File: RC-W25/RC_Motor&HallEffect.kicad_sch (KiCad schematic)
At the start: 10 parts, among them P1 CONN HEADER SMD R/A 2POS 2MM, Q1 NMOS, U3 TMAG5253, U4 TMAG5253, U6 PTS645SM43SMTR92LFS

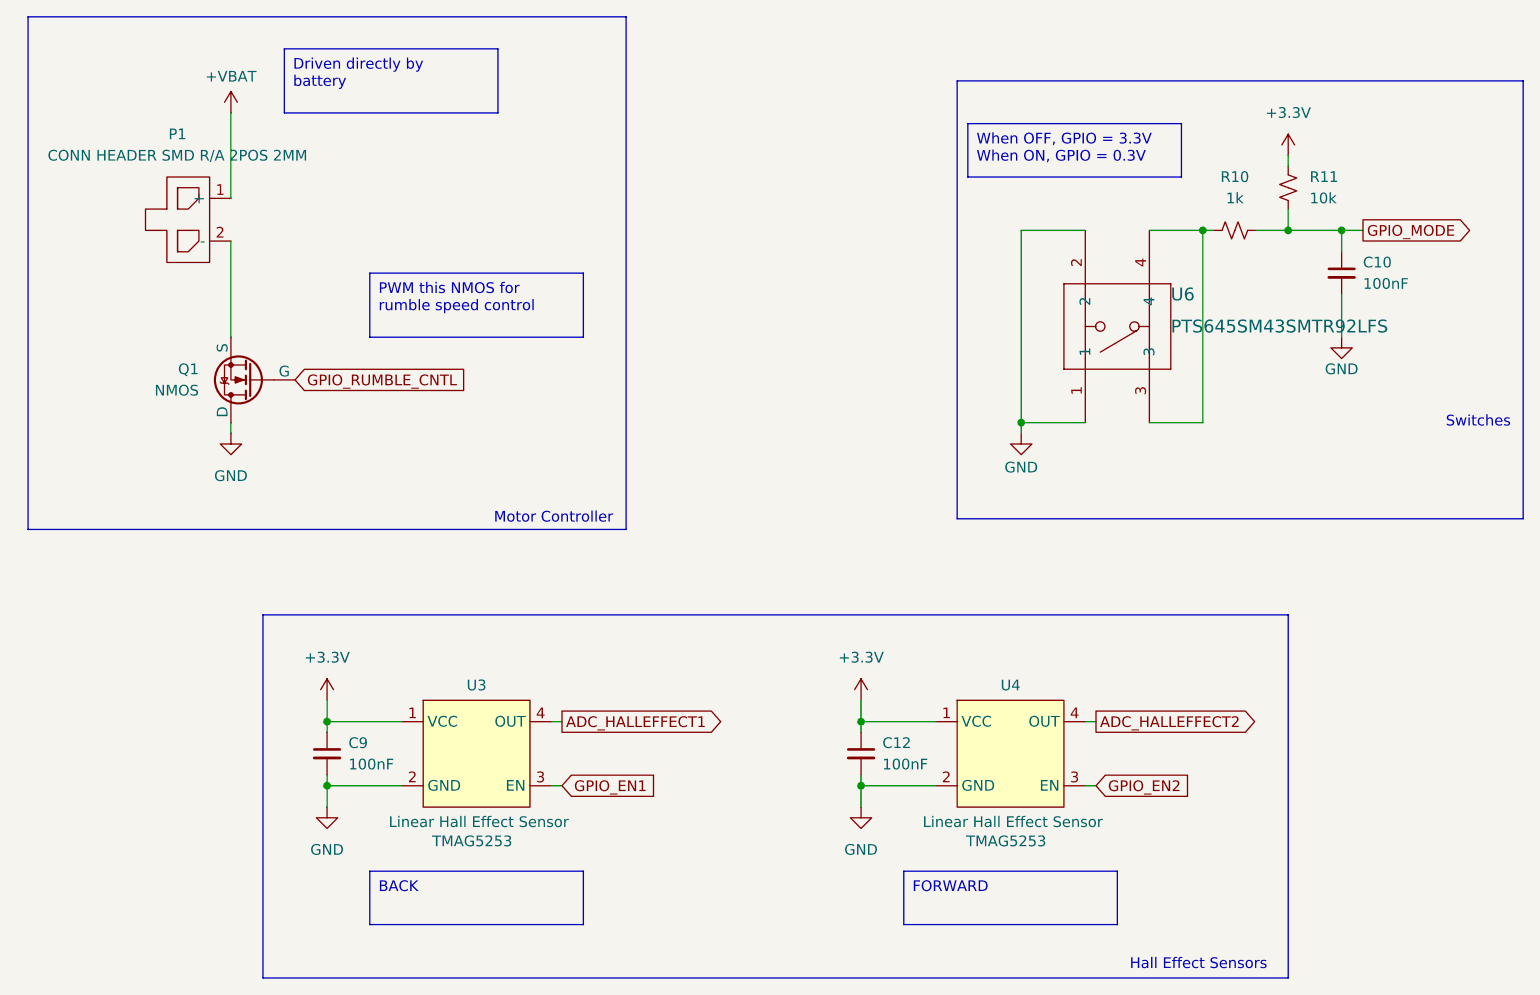
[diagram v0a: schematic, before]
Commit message: Almost Finalized Schematic
Still need to spec out buttons and jst conn
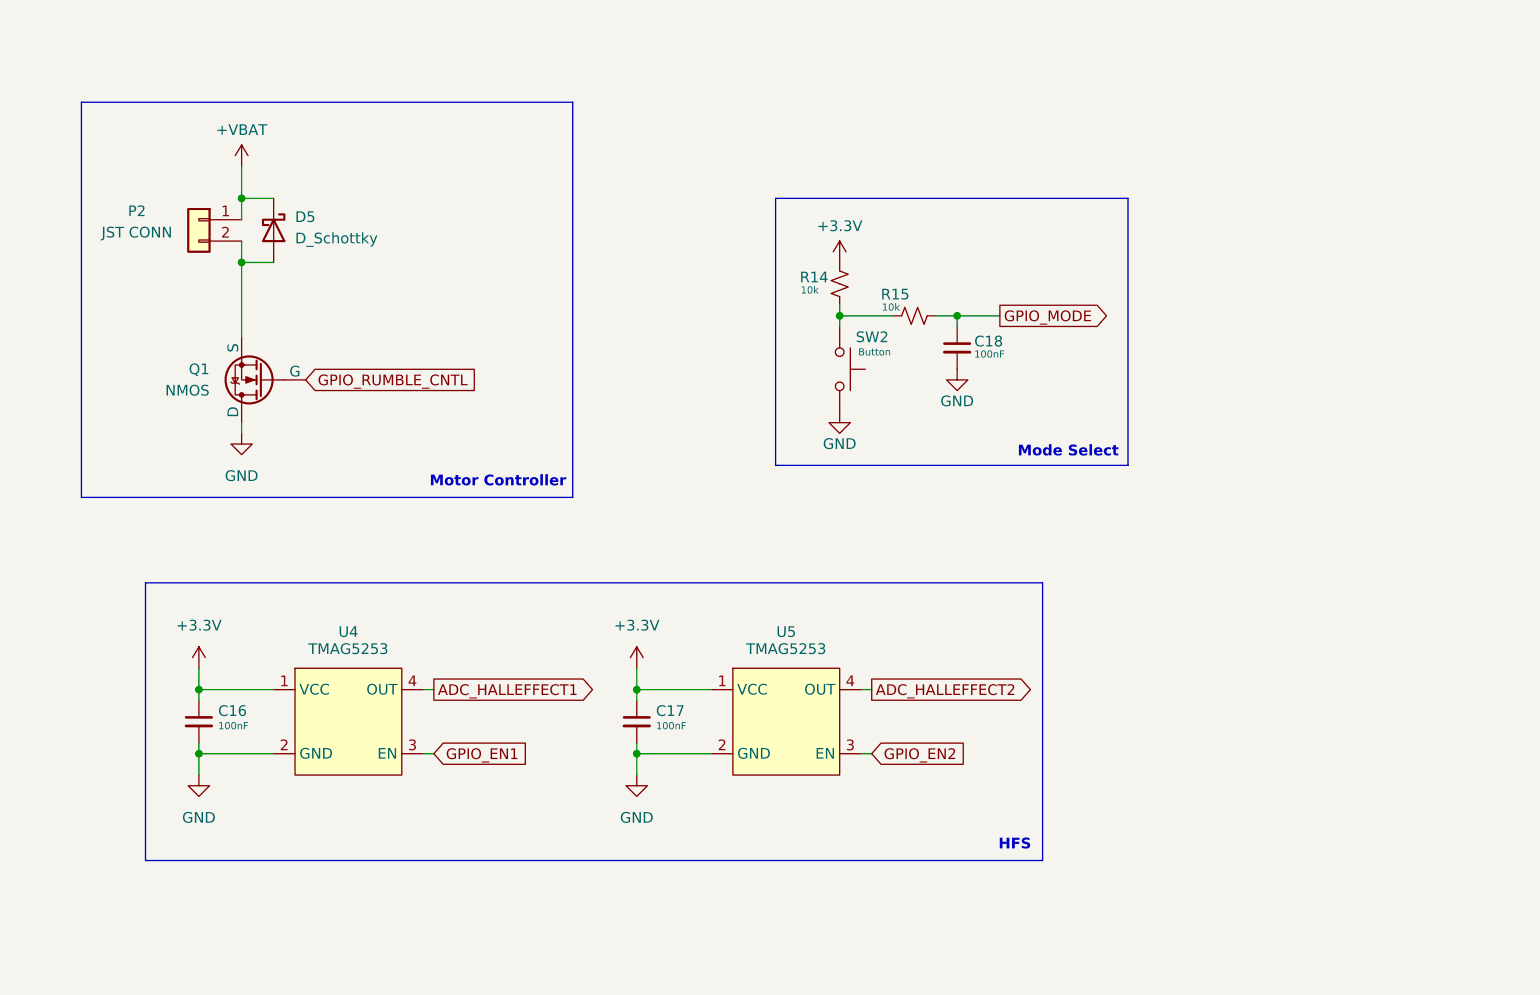
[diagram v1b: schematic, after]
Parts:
- removed C10, C12: 100nF, Capacitor_SMD:C_0603_1608Metric, symbol Device:C_Small
- removed P1: CONN HEADER SMD R/A 2POS 2MM, Library:CONN02_502352_MOL, symbol New_Library:DuraClik_CONN_HEADER_SMD_R/A_2POS_2MM
- removed R10: 1k, Resistor_SMD:R_0603_1608Metric, symbol Device:R_Small_US
- removed R11: 10k, Resistor_SMD:R_0603_1608Metric, symbol Device:R_Small_US
- removed U4: TMAG5253, Library:X2SON4_DMR_TEX-M, symbol New_Library_0:TMAG5253_Linear_Hall_Effect_Sensor
- removed U6: PTS645SM43SMTR92LFS, Library:SWITCH_43SMTR92LFS, symbol New_Library_5:PTS645SM43SMTR92LFS
- added C17, C18: 100nF, Capacitor_SMD:C_0402_1005Metric, symbol Device:C_Small
- added D5: D_Schottky, Diode_SMD:D_SOD-123, symbol Device:D_Schottky
- added P2: JST CONN, Library:CONN02_502352_MOL, symbol Connector_Generic:Conn_01x02
- added R14, R15: 10k, Resistor_SMD:R_0402_1005Metric, symbol Device:R_Small_US
- added SW2: Button, symbol Switch:SW_Push
- added U5: TMAG5253, Library:X2SON4_DMR_TEX-M, symbol New_Library_0:TMAG5253_Linear_Hall_Effect_Sensor
- C16: renamed from C9; footprint Capacitor_SMD:C_0603_1608Metric -> Capacitor_SMD:C_0402_1005Metric; LCSC# (none) -> C22435938
- U4: renamed from U3; LCSC# (none) -> C22445458
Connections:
- net +3.3V: now also C17.1, R14.1, U5.1 (VCC)
- net +VBAT: now also D5.1 (K), P2.1 (Pin_1)
- net ADC_HALLEFFECT2: now also U5.4 (OUT)
- net GND: now also C17.2, C18.2, SW2.2, U5.2 (GND)
- net GPIO_EN2: now also U5.3 (EN)
- net GPIO_MODE: now also C18.1, R15.2
- net at Q1.3 (S): now also D5.2 (A), P2.2 (Pin_2)
- new net: R14.2, R15.1, SW2.1
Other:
- note added: "HFS"
- note added: "Mode Select"
- note removed: "Hall Effect Sensors"
- note removed: "Switches"
- moved on the sheet: C16, Q1, U4
